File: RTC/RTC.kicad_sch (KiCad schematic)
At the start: 16 parts, among them J1 Rasberry_to_stm, J10 Servo1, J11 Power 12V, J2 Encoder R, J3 motor R, J4 Encoder L, J5 motor L, J6 Servo1, J7 Servo2, J8 Servo3, J9 Servo4, U2 L298N

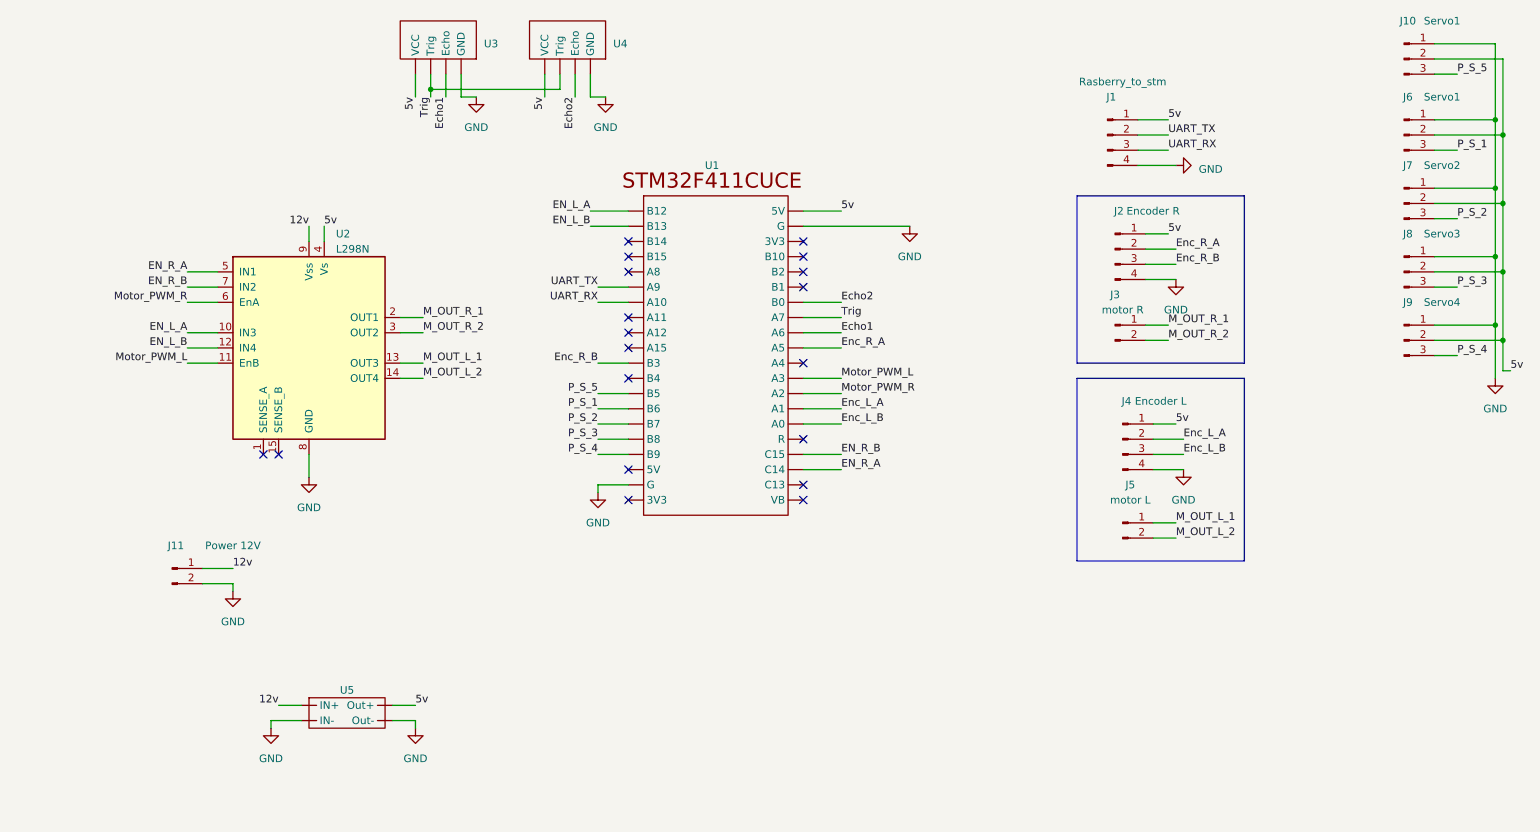
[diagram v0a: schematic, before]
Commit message: Work with PID on velocity
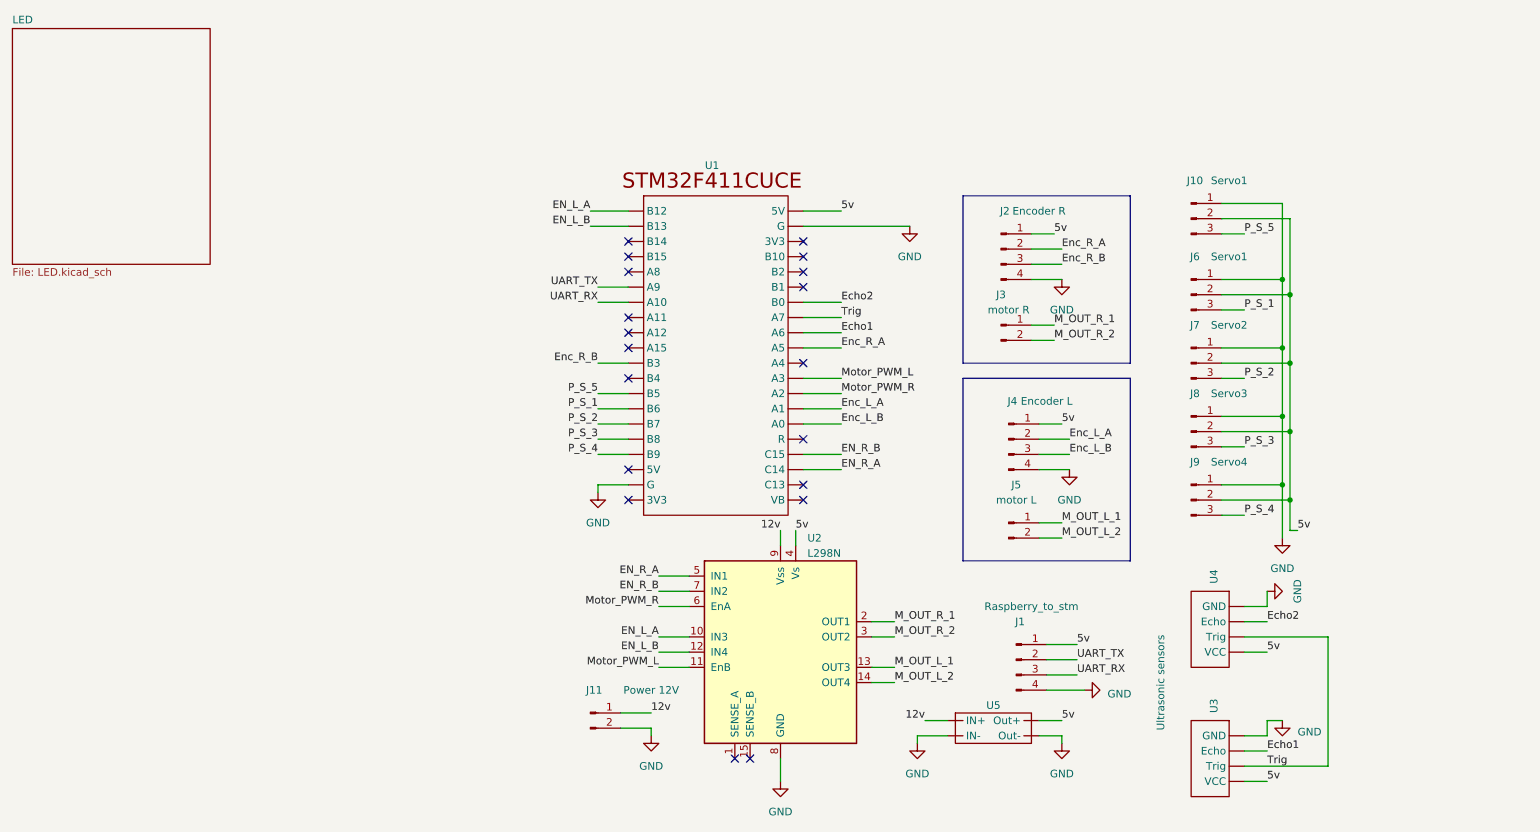
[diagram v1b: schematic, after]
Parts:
- J1: value Rasberry_to_stm -> Raspberry_to_stm
- U3: value ~ -> Ultrasonic sensors
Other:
- added sheet LED (LED.kicad_sch)
- moved on the sheet: J1, J10, J11, J2, J3, J4, J5, J6, J7, J8, J9, U2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
